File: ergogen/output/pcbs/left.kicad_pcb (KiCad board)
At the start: 2 copper layers, 130.6 x 90.5 mm, 59 parts

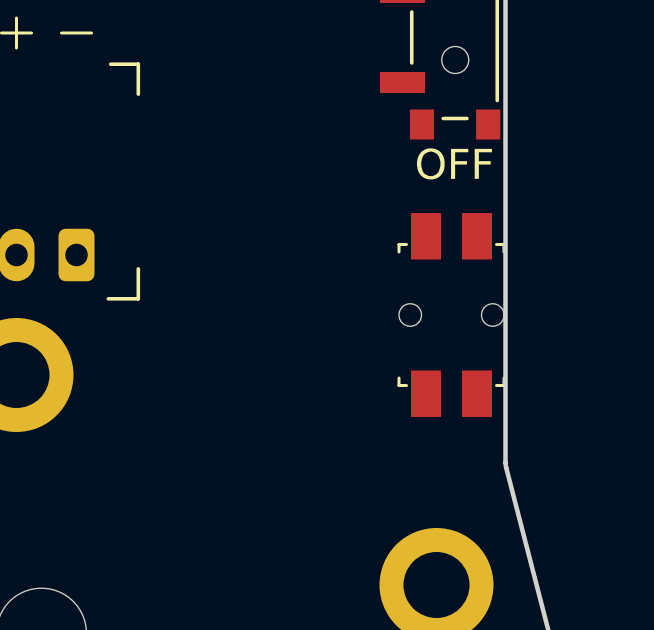
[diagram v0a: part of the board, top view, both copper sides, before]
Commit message: add: v2 gerbers
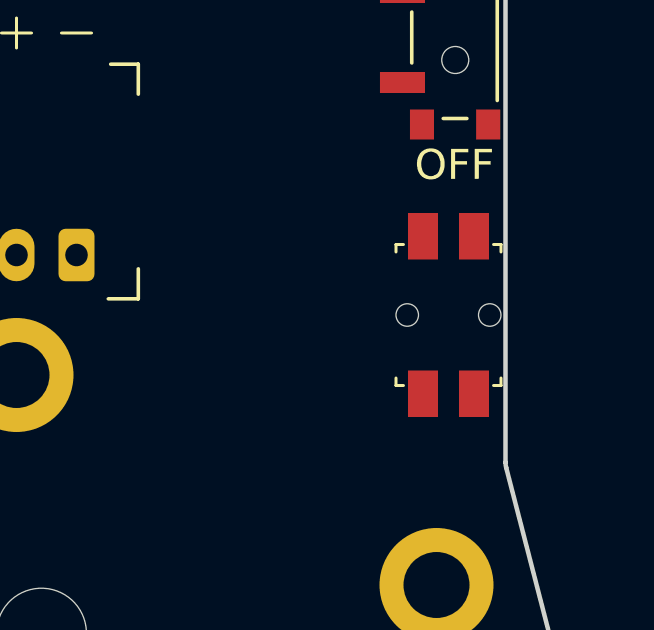
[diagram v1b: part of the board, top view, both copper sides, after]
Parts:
- moved RST1 0.10 mm to (286.2, 169.3)
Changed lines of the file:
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@@
   (footprint "ceoloide:reset_switch_smd_side"
     (layer "F.Cu")
-    (at 286.3 169.3 -90)
+    (at 286.2 169.3 -90)
     (property "Reference" "RST1"
       (at 0 0 -90)
